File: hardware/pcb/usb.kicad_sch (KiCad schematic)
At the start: 39 parts, among them J800 USB_C_Receptacle, U800 USBLC6-2P6, U801 FUSB302BMPX, U802 CBTL08GP053, U803 TC358777, X800 19.2MHz

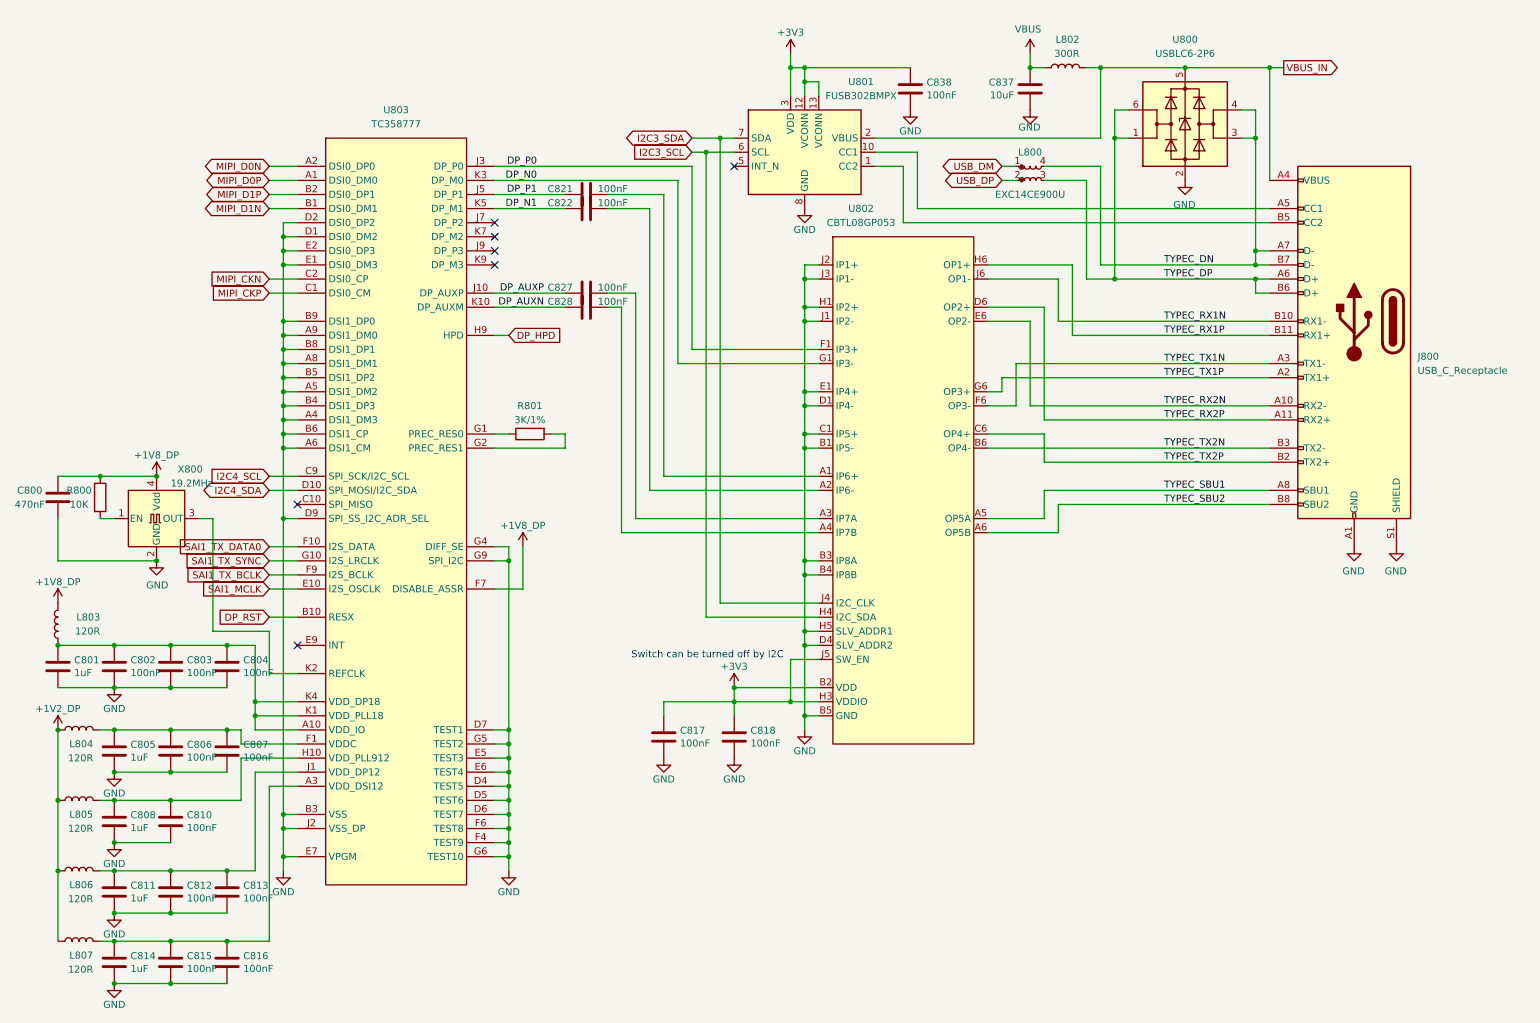
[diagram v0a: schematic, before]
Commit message: - PCB: prepare for r0p4
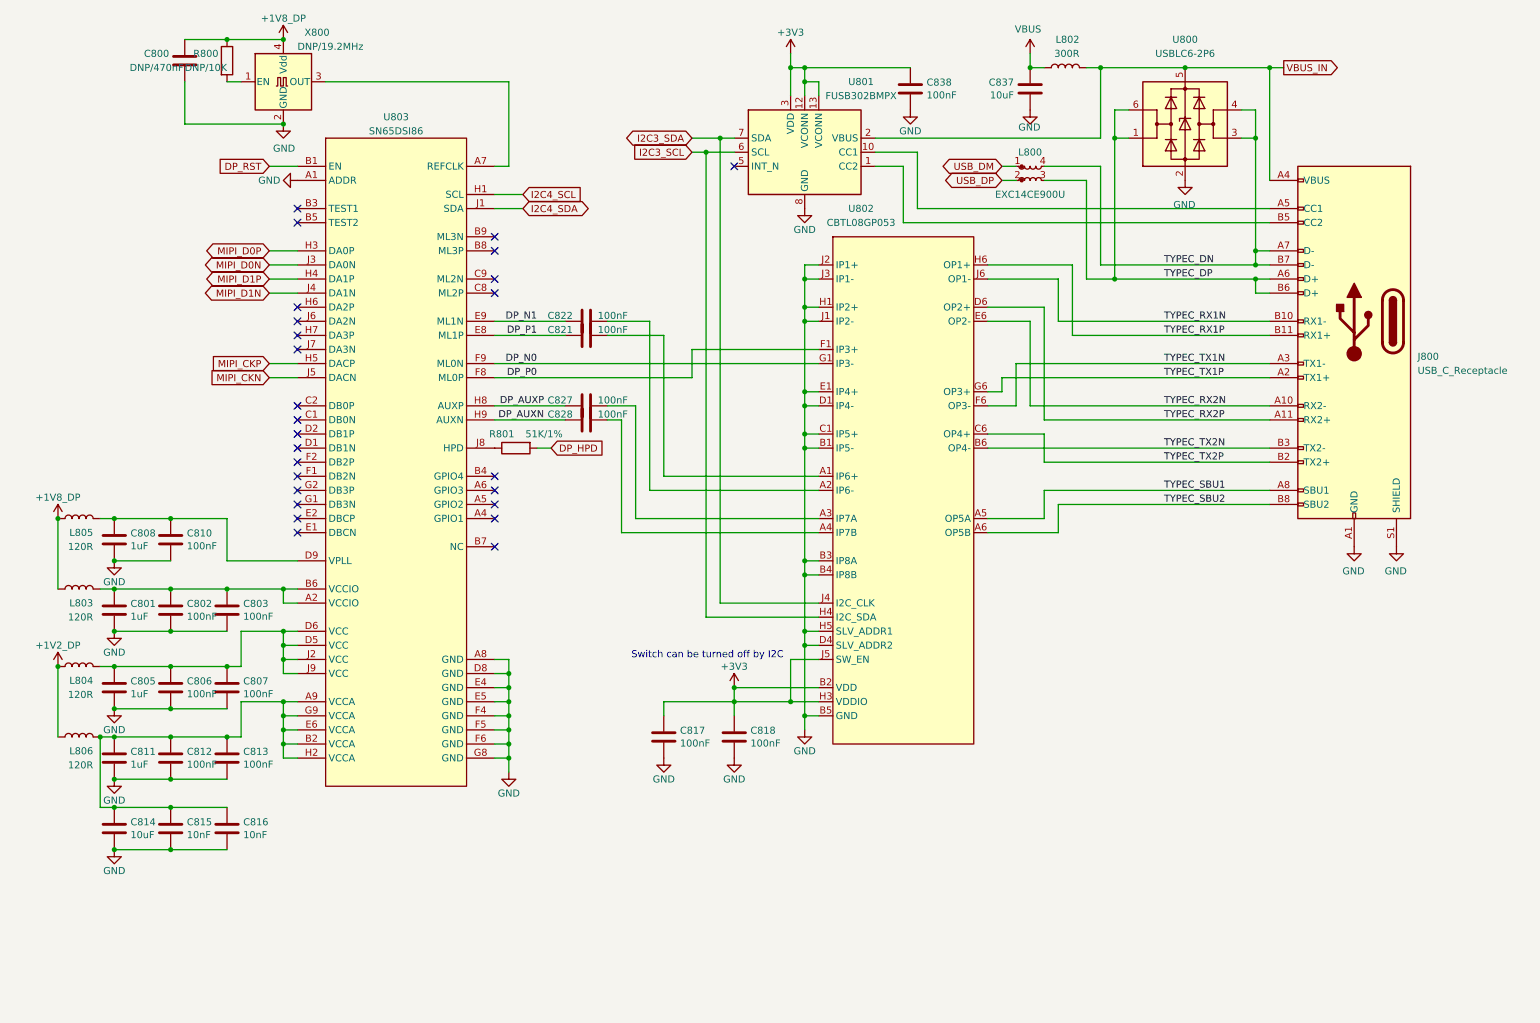
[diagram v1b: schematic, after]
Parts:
- removed C804: 100nF, Capacitor_SMD:C_0201_0603Metric, symbol Device:C
- removed L807: 120R, Inductor_SMD:L_0402_1005Metric, symbol Device:L
- removed U803: TC358777, footprint:BGA-80_10x10_7.0x7.0mm, symbol symbols:TC358777
- added U803: SN65DSI86, footprint:BGA-64_9x9_5.0x5.0mm, symbol symbols:SN65DSI86
- C800: value 470nF -> DNP/470nF
- C814: value 1uF -> 10uF
- C815, C816: value 100nF -> 10nF
- R800: value 10K -> DNP/10K
- R801: value 3K/1% -> 51K/1%
- X800: value 19.2MHz -> DNP/19.2MHz
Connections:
- net +1V2_DP: no longer L805.1
- net +1V8_DP: now also L803.1, L805.1; no longer L803.2
- net DP_AUXN: now also U803.H9 (AUXN)
- net DP_AUXP: now also U803.H8 (AUXP)
- net DP_HPD: now also R801.2
- net DP_N0: now also U803.F9 (ML0N)
- net DP_N1: now also U803.E9 (ML1N)
- net DP_P0: now also U803.F8 (ML0P)
- net DP_P1: now also U803.E8 (ML1P)
- net DP_RST: now also U803.B1 (EN)
- net GND: now also U803.A1 (ADDR), U803.A8 (GND), U803.D8 (GND), U803.E4 (GND), U803.E5 (GND), U803.F4 (GND), U803.F5 (GND), U803.F6 (GND), U803.G8 (GND)
- net I2C4_SCL: now also U803.H1 (SCL)
- net I2C4_SDA: now also U803.J1 (SDA)
- net MIPI_CKN: now also U803.J5 (DACN)
- net MIPI_CKP: now also U803.H5 (DACP)
- net MIPI_D0N: now also U803.J3 (DA0N)
- net MIPI_D0P: now also U803.H3 (DA0P)
- net MIPI_D1N: now also U803.J4 (DA1N)
- net MIPI_D1P: now also U803.H4 (DA1P)
- net at C801.1, C802.1, C803.1: now also L803.2, U803.A2 (VCCIO), U803.B6 (VCCIO); no longer L803.1
- net at C805.1, C806.1, C807.1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: now also U803.D5 (VCC), U803.D6 (VCC), U803.J2 (VCC), U803.J9 (VCC)
- net at C808.1, C810.1, L805.2: now also U803.D9 (VPLL)
- net at C814.1, C815.1, C816.1: now also C811.1, C812.1, C813.1, L806.2, U803.A9 (VCCA), U803.B2 (VCCA), U803.E6 (VCCA), U803.G9 (VCCA), U803.H2 (VCCA)
- net at R801.1: now also U803.J8 (HPD)
- net at X800.3 (OUT): now also U803.A7 (REFCLK)
- no-connect marks 7 -> 26
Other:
- moved on the sheet: C800, C801, C802, C803, C805, C806, C807, C808, C810, C811, C812, C813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
